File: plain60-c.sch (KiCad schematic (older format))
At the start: 176 parts, among them J1 HRO-TYPE-C-31-M-12, J2 ISP, K1 KEYSW, K10 KEYSW, K11 KEYSW, K12 KEYSW, K13 KEYSW, K14 KEYSW, K15 KEYSW, K15-1 KEYSW, K16 KEYSW, K17 KEYSW, K18 KEYSW, K19 KEYSW, K2 KEYSW, K20 KEYSW, K21 KEYSW, K22 KEYSW, K23 KEYSW, K24 KEYSW, K25 KEYSW, K26 KEYSW, K27 KEYSW, K28 KEYSW, K29 KEYSW, K3 KEYSW, K31 KEYSW, K31-1 KEYSW, K32 KEYSW, K33 KEYSW, K34 KEYSW, K35 KEYSW, K36 KEYSW, K37 KEYSW, K38 KEYSW, K39 KEYSW, K4 KEYSW, K40 KEYSW, K41 KEYSW, K42 KEYSW, K43 KEYSW, K44 KEYSW, K44-1 KEYSW, K46 KEYSW, K46-1 KEYSW, K47 KEYSW, K48 KEYSW, K49 KEYSW, K5 KEYSW, K50 KEYSW, K51 KEYSW, K52 KEYSW, K53 KEYSW, K54 KEYSW, K55 KEYSW, K56 KEYSW, K57 KEYSW, K58 KEYSW, K58-1 KEYSW, K59 KEYSW, K6 KEYSW, K61 KEYSW, K61-1 KEYSW, K62 KEYSW, K62-1 KEYSW, K63 KEYSW, K63-1 KEYSW, K67 KEYSW, K67-1 KEYSW, K7 KEYSW, K71 KEYSW, K72 KEYSW, K72-1 KEYSW, K73 KEYSW, K73-1 KEYSW, K74 KEYSW, K74-1 KEYSW, K8 KEYSW, K9 KEYSW, SW1 SW_PUSH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

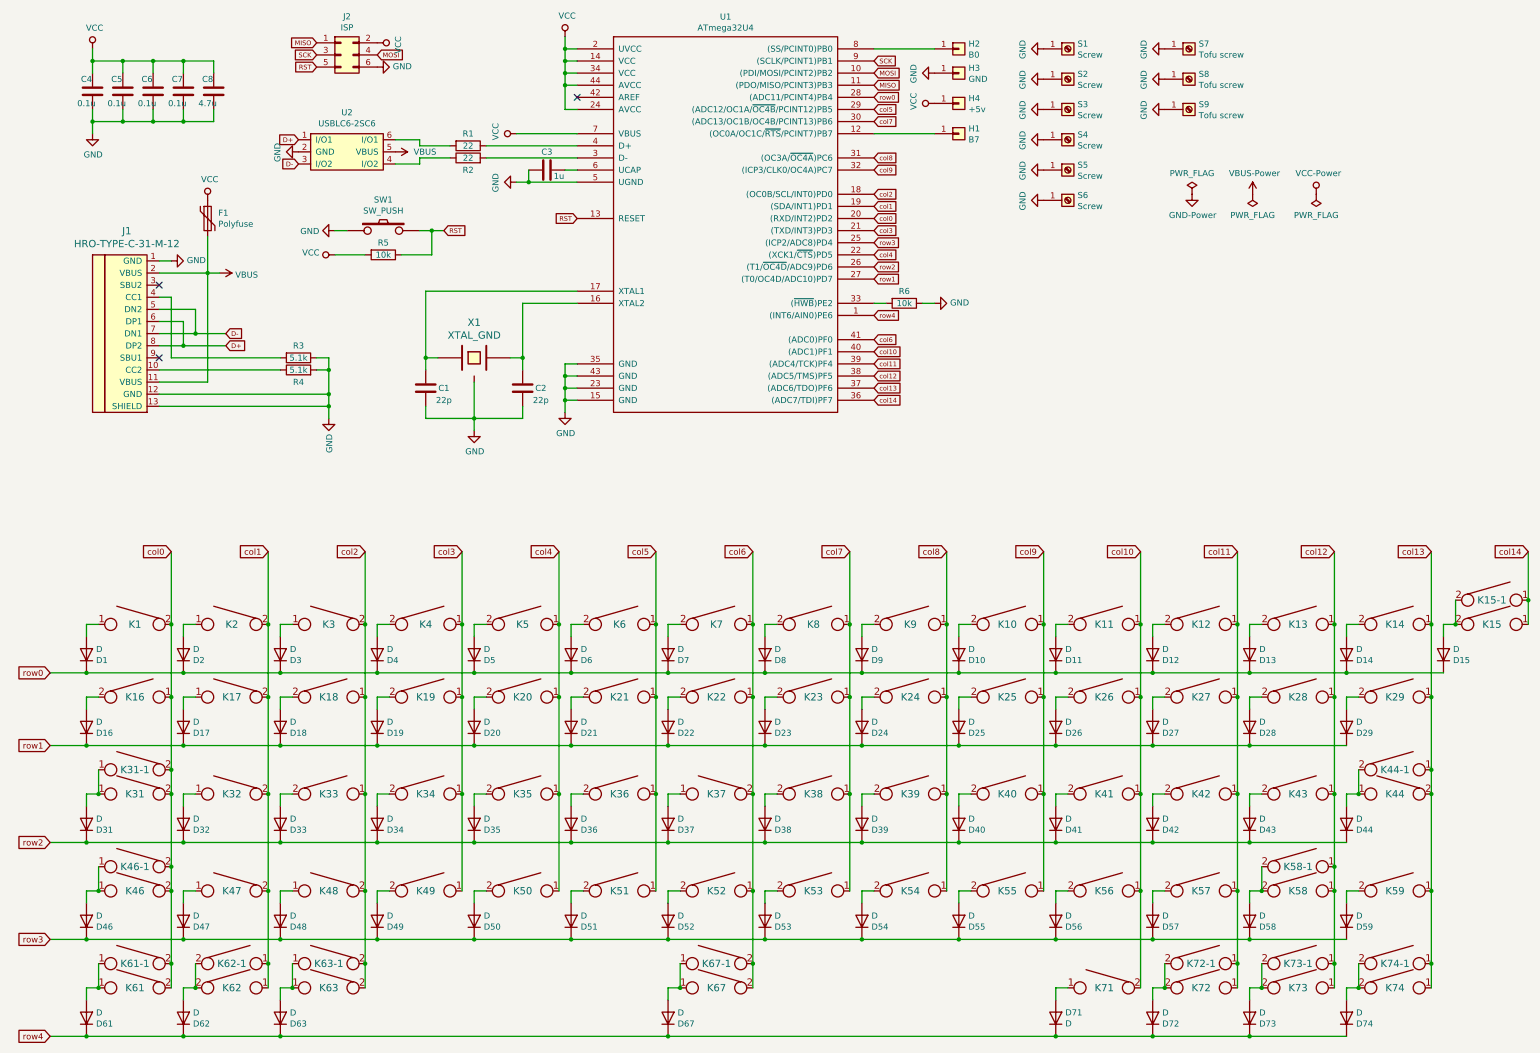
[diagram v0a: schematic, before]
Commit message: remove components.
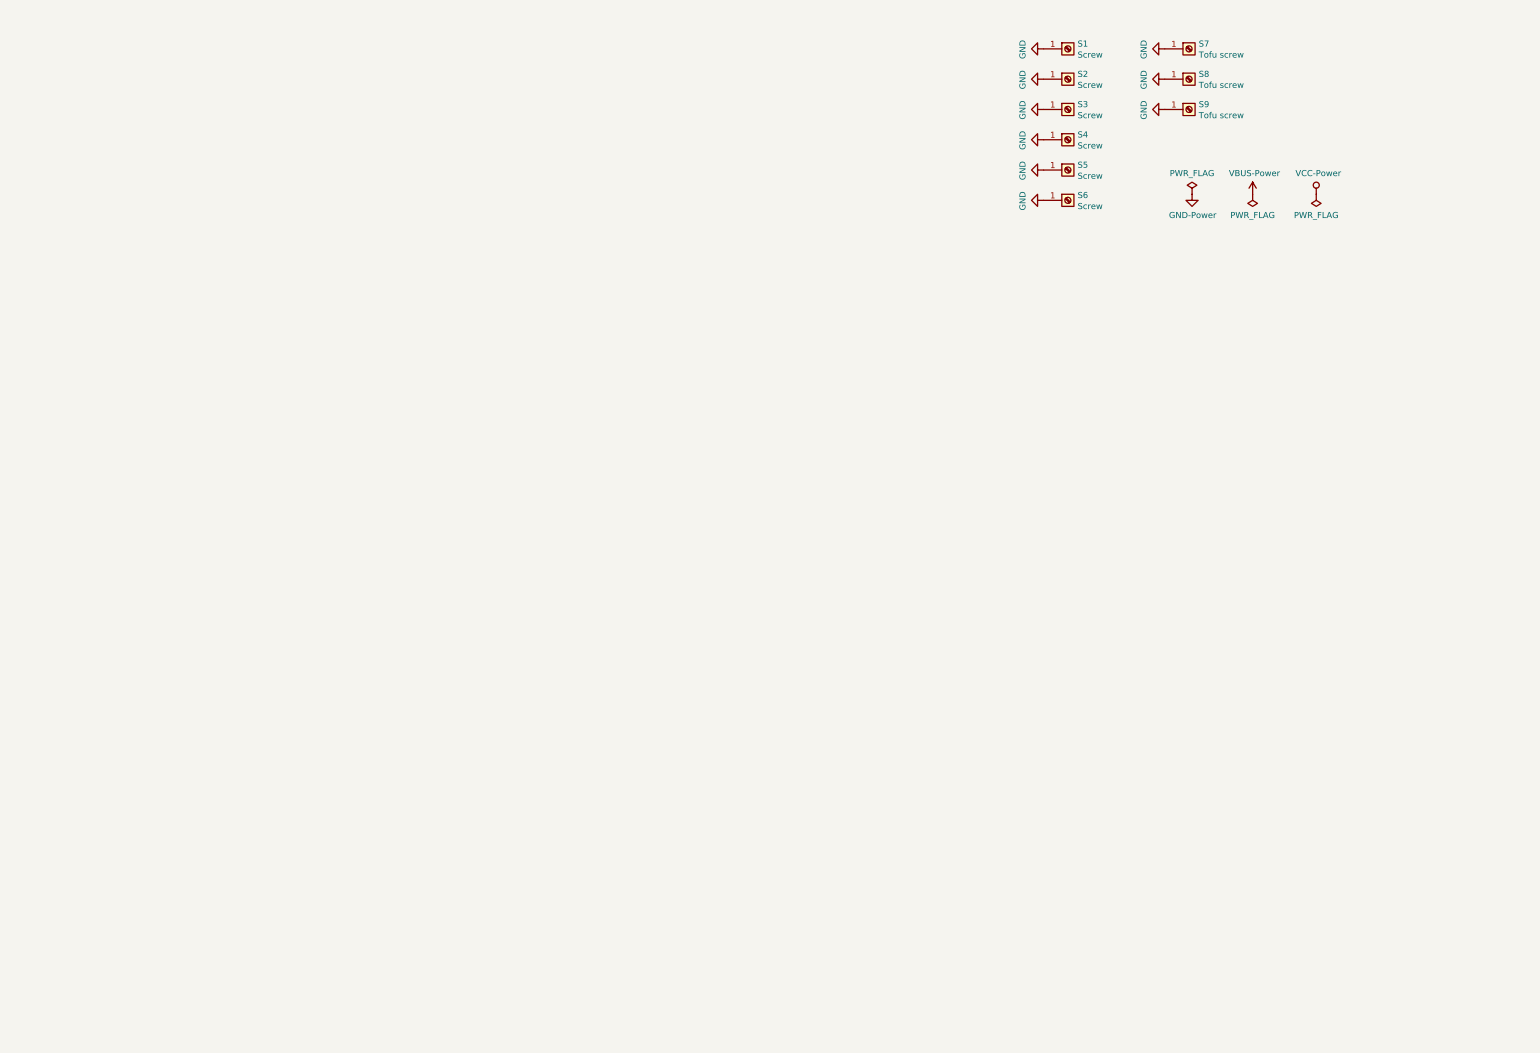
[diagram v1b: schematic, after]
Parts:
- removed C1, C2: 22p, Keeb_components:C_0805, symbol Device:C
- removed C3: 1u, Keeb_components:C_0805, symbol Device:C
- removed C4, C5, C6, C7: 0.1u, Keeb_components:C_0805, symbol Device:C
- removed C8: 4.7u, Keeb_components:C_0805, symbol Device:C
- removed D1, D10, D11, D12, D13, D14, D15, D16, D17, D18, D19, D2, D20, D21, D22, D23, D24, D25, D26, D27, D28, D29, D3, D31, D32, D33, D34, D35, D36, D37, D38, D39, D4, D40, D41, D42, D43, D44, D46, D47, D48, D49, D5, D50, D51, D52, D53, D54, D55, D56, D57, D58, D59, D6, D61, D62, D63, D67, D7, D71, D72, D73, D74, D8, D9: D, Keeb_components:D_0805, symbol Device:D
- removed F1: Polyfuse, Keeb_components:R_0805, symbol Device:Polyfuse
- removed H1: B7, footprints:free_pin, symbol Connector_Generic:Conn_01x01
- removed H2: B0, footprints:free_pin, symbol Connector_Generic:Conn_01x01
- removed H3: GND, footprints:free_pin, symbol Connector_Generic:Conn_01x01
- removed H4: +5v, footprints:free_pin, symbol Connector_Generic:Conn_01x01
- removed J1: HRO-TYPE-C-31-M-12, Keeb_components:HRO-TYPE-C-31-M-12, symbol plain60-c-rescue:HRO-TYPE-C-31-M-12-Type-C
- removed J2: ISP, Keeb_components:isp_standard, symbol Connector_Generic:Conn_02x03_Odd_Even
- removed K1, K10, K11, K12, K13, K14, K15-1, K17, K18, K19, K2, K20, K21, K22, K23, K24, K25, K26, K27, K28, K3, K32, K33, K34, K35, K36, K37, K38, K39, K4, K40, K41, K42, K43, K47, K48, K49, K5, K50, K51, K52, K53, K54, K55, K56, K57, K59, K6, K62-1, K7, K73-1, K8, K9: KEYSW, Keeb_switches:CHERRY_PLATE_100H, symbol plain60-c-rescue:KEYSW-keyboard_parts
- removed K15: KEYSW, Keeb_switches:CHERRY_PCB_200H, symbol plain60-c-rescue:KEYSW-keyboard_parts
- removed K16, K29, K61-1, K63-1, K72-1, K74-1: KEYSW, Keeb_switches:CHERRY_PLATE_150H, symbol plain60-c-rescue:KEYSW-keyboard_parts
- removed K31, K58-1: KEYSW, Keeb_switches:CHERRY_PLATE_175H, symbol plain60-c-rescue:KEYSW-keyboard_parts
- removed K31-1, K46-1, K61, K62, K63, K71, K72, K73, K74: KEYSW, Keeb_switches:CHERRY_PLATE_125H, symbol plain60-c-rescue:KEYSW-keyboard_parts
- removed K44, K46: KEYSW, Keeb_switches:CHERRY_PCB_225H, symbol plain60-c-rescue:KEYSW-keyboard_parts
- removed K44-1: KEYSW, Keeb_switches:CHERRY_PCB_200H_V, symbol plain60-c-rescue:KEYSW-keyboard_parts
- removed K58: KEYSW, Keeb_switches:CHERRY_PCB_275H, symbol plain60-c-rescue:KEYSW-keyboard_parts
- removed K67: KEYSW, Keeb_switches:CHERRY_PCB_625H_F, symbol plain60-c-rescue:KEYSW-keyboard_parts
- removed K67-1: KEYSW, Keeb_switches:CHERRY_PCB_700H_F, symbol plain60-c-rescue:KEYSW-keyboard_parts
- removed R1, R2: 22, Keeb_components:R_0805, symbol Device:R
- removed R3, R4: 5.1k, Keeb_components:R_0805, symbol Device:R
- removed R5, R6: 10k, Keeb_components:R_0805, symbol Device:R
- removed SW1: SW_PUSH, Button_Switch_SMD:SW_SPST_TL3342, symbol plain60-c-rescue:SW_PUSH-keyboard_parts
- removed U1: ATmega32U4, Keeb_components:ATMEGA32U4, symbol plain60-c-rescue:ATmega32U4-atmel
- removed U2: USBLC6-2SC6, Keeb_components:USBLC6-2SC6, symbol plain60-c-rescue:USBLC6-2SC6-keyboard_parts
- removed X1: XTAL_GND, Keeb_components:crystal_FA238-TSX3225, symbol plain60-c-rescue:XTAL_GND-keyboard_parts
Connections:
- no-connect marks 3 -> 0
